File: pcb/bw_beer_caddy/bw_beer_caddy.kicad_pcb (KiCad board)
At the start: 2 copper layers, 70 x 64 mm, 38 parts, among them J1 Screw_Terminal_01x06, J3 Screw_Terminal_01x03, J4 Screw_Terminal_01x03, J5 Conn_01x03_Female, J6 Conn_01x03_Female, J7 Conn_02x04_Top_Bottom, J8 Conn_02x04_Top_Bottom, J9 Screw_Terminal_01x06, K1 G5LE-1, Q1 2N3904, Q2 FQP27P06, Q3 2N7000, Q4 2N3904, Q5 2N7000, U1 ina219_breakout, U2 LM2575-5.0BT, U3 LM2575-12BT, U4 LM2575-12BT, U5 LM2575-12BT, U6 SEN-13879

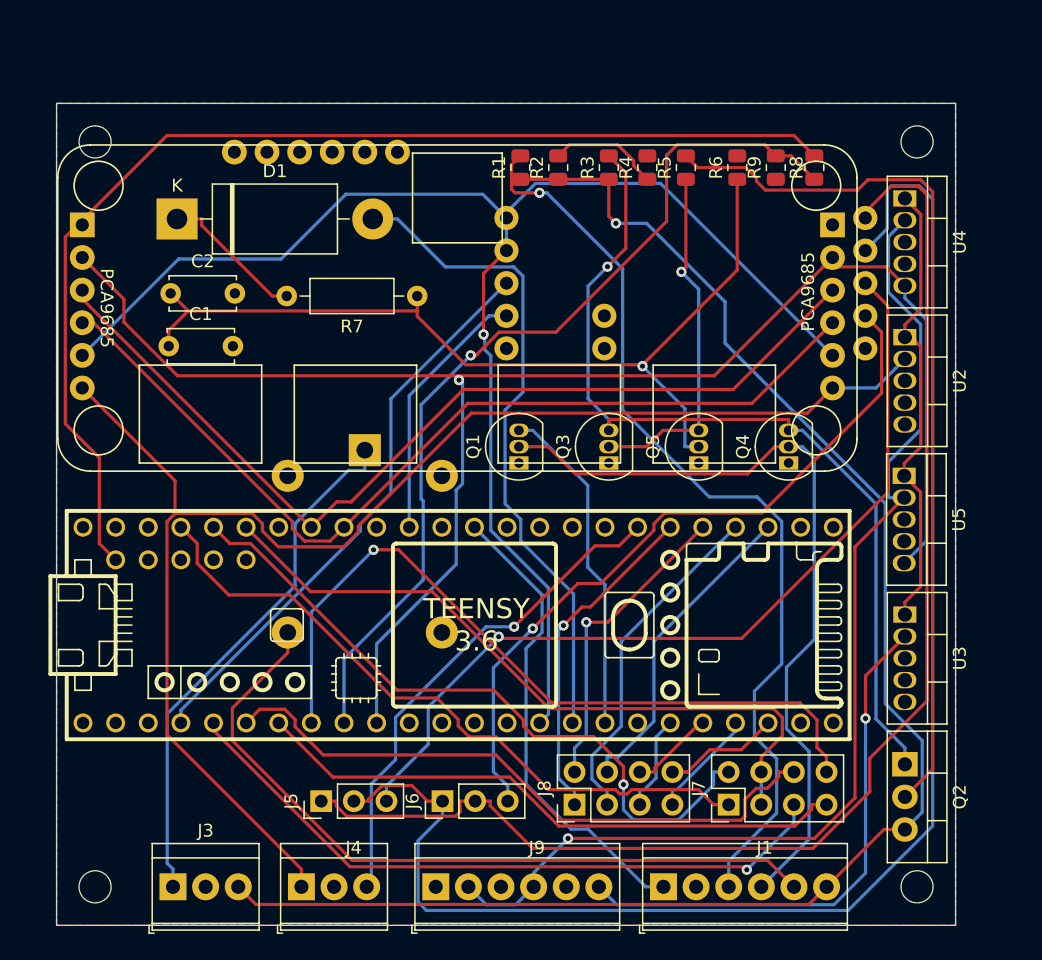
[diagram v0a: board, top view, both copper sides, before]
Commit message: bw_bcause rev 00 release
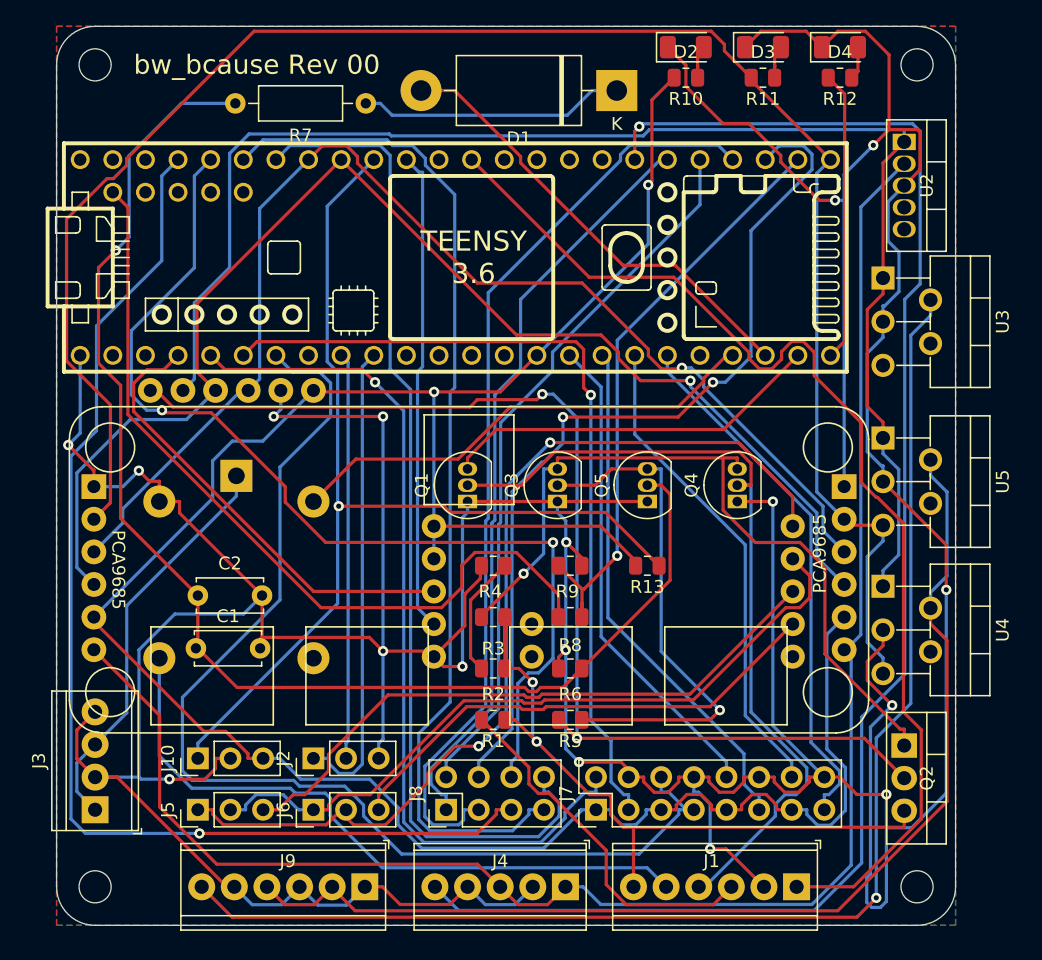
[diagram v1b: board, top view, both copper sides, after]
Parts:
- added D2: LED, LED_SMD:LED_1206_3216Metric, F.Cu at (149.0, 45.6)
- added D3: LED, LED_SMD:LED_1206_3216Metric, F.Cu at (155.0, 45.6)
- added D4: LED, LED_SMD:LED_1206_3216Metric, F.Cu at (161.0, 45.6)
- added J10: Conn_01x03_Female, Connector_PinHeader_2.54mm:PinHeader_1x03_P2.54mm_Vertical, F.Cu at (111.0, 101.0)
- added J2: Conn_01x03_Female, Connector_PinHeader_2.54mm:PinHeader_1x03_P2.54mm_Vertical, F.Cu at (120.0, 101.0)
- added R10: 10K, Resistor_SMD:R_0805_2012Metric, F.Cu at (149.0, 48.0)
- added R11: 10K, Resistor_SMD:R_0805_2012Metric, F.Cu at (155.0, 48.0)
- added R12: 10K, Resistor_SMD:R_0805_2012Metric, F.Cu at (161.0, 48.0)
- added R13: 10K, Resistor_SMD:R_0805_2012Metric, F.Cu at (146.0, 86.0)
- J3: value Screw_Terminal_01x03 -> Screw_Terminal_01x04; footprint TerminalBlock_TE-Connectivity:TerminalBlock_TE_282834-3_1x03_P2.54mm_Horizontal -> TerminalBlock_TE-Connectivity:TerminalBlock_TE_282834-4_1x04_P2.54mm_Horizontal
- J4: value Screw_Terminal_01x03 -> Screw_Terminal_01x05; footprint TerminalBlock_TE-Connectivity:TerminalBlock_TE_282834-3_1x03_P2.54mm_Horizontal -> TerminalBlock_TE-Connectivity:TerminalBlock_TE_282834-5_1x05_P2.54mm_Horizontal
- J7: value Conn_02x04_Top_Bottom -> Conn_02x08_Top_Bottom; footprint Connector_PinHeader_2.54mm:PinHeader_2x04_P2.54mm_Vertical -> Connector_PinHeader_2.54mm:PinHeader_2x08_P2.54mm_Vertical
- R8: value 6K -> 10K
- U3, U4, U5: value LM2575-12BT -> LM2576TV-012G; footprint Package_TO_SOT_THT:TO-220-5_Vertical -> Package_TO_SOT_THT:TO-220-5_P3.4x3.7mm_StaggerOdd_Lead3.8mm_Vertical
- moved R5 43.9 mm to (140.0, 98.0), turned to 180 degrees
- moved R1 43.1 mm to (134.0, 98.0), turned to 180 degrees
- moved R6 41.1 mm to (140.0, 94.0), turned to 180 degrees
- moved R8 39.8 mm to (140.0, 90.0), turned to 180 degrees
- moved R2 39.3 mm to (134.0, 94.0), turned to 180 degrees
- moved R3 36.1 mm to (134.0, 90.0), turned to 180 degrees
- moved D1 35.7 mm to (143.6, 49.0), turned to 180 degrees
- moved R9 34.9 mm to (140.0, 86.0), turned to 180 degrees
- moved R4 33.2 mm to (134.0, 86.0), turned to 180 degrees
- moved U1 31.1 mm to (126.7, 75.1), turned to 180 degrees
- moved U4 30.2 mm to (164.3, 87.6)
- moved U$2 28.6 mm to (129.8, 62.0)
- moved U3 26.3 mm to (164.3, 63.6)
- moved U6 24.7 mm to (143.3, 88.0)
- moved C1 23.6 mm to (110.8, 92.4)
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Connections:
- J3 pad 3: /MAIN_SWT_OUT -> Net-(J3-Pad1)
- J4 pad 3: /LED_RING -> +5V
- J7 pad 1: /M1_EA -> +3.3V
- J7 pad 2: /M1_EB -> /M1_EA
- J7 pad 3: /M2_EA -> /M1_EB
- J7 pad 4: /M2_EA -> GND
- J7 pad 5: /M3_EA -> +3.3V
- J7 pad 6: /M3_EB -> /M2_EA
- J7 pad 7: /M4_EA -> /M2_EA
- J7 pad 8: /M4_EB -> GND
- U$2 pad 17/A3: unconnected-(U$2-Pad17/A3) -> /HALL_EFFECT_SNS
- U$2 pad 20/A6: /M2_EB -> /M4_DR2
- U$2 pad 21/A7: /M2_EA -> /M4_DR1
- U$2 pad 22/A8: /M1_EB -> /M3_DR2
- U$2 pad 23/A9: /M1_EA -> /M3_DR1
- U$2 pad 24: /UNLATCH -> /M3_EA
- U$2 pad 25: /LATCH_STAT -> /M3_EB
- U$2 pad 26: unconnected-(U$2-Pad26) -> /M4_EA
- U$2 pad 27: /M3_DR1 -> /M4_EB
- U$2 pad 28: /M3_DR2 -> unconnected-(U$2-Pad28)
- U$2 pad 29: /M4_DR1 -> /CHARGE_RELAY_CTRL
- U$2 pad 3/CANTX: /M3_EA -> /M1_EA
- U$2 pad 30: /M4_DR2 -> /UNLATCH
- U$2 pad 31/A12: unconnected-(U$2-Pad31/A12) -> /LATCH_STAT
- U$2 pad 32/A13: unconnected-(U$2-Pad32/A13) -> /STATUS_LED
- U$2 pad 33/A14: /RX_JETSON -> /MOTOR_ENABLE
- U$2 pad 34/A15: /TX_JETSON -> /USB_SENSE
- U$2 pad 4/CANRX: /M3_EB -> /M1_EB
- U$2 pad 5: /M4_EA -> /M2_EA
- U$2 pad 6: /M4_EB -> /M2_EB
- U$2 pad 7: /USB_SENSE -> /RX_JETSON
- U$2 pad 8: /MOTOR_ENABLE -> /TX_JETSON
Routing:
- net GND: track 0.00 -> 465.3 mm, vias 0 -> 17
- net /M3_DR1: track 7.56 -> 90.5 mm, vias 0 -> 1
- net /HALL_EFFECT_SNS: track 0.00 -> 80.8 mm, vias 0 -> 1
- net /LED_RING: track 39.1 -> 119.3 mm
- net +3.3V: track 113.7 -> 191.3 mm, vias 1 -> 2
- net VDD: track 36.0 -> 111.7 mm
- net /M3_DR2: track 6.68 -> 79.2 mm, vias 0 -> 2
- net /M4_DR1: track 8.61 -> 80.0 mm
- net /MAIN_SWT_OUT: track 124.5 -> 54.7 mm, vias 1 -> 2
- net /M4_DR2: track 9.03 -> 78.6 mm
- net /E-: track 118.0 -> 57.1 mm
- net +12L: track 42.1 -> 102.4 mm
- net /BUTTON_LED: track 36.7 -> 87.0 mm
- net /M2_DR1: track 26.9 -> 72.8 mm
- net /M2_DR2: track 24.8 -> 69.5 mm, vias 0 -> 2
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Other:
- board size 70 x 64 mm -> 70 x 70 mm
- board text added: "Ben Warwick 2022"
- board text added: "bw_bcause Rev 00"
